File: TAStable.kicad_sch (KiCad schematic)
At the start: 12 parts, among them J1 Conn_01x06_Pin, U1 74HCT1G04, U2 CS2300-CP, U3 74LVC1G14

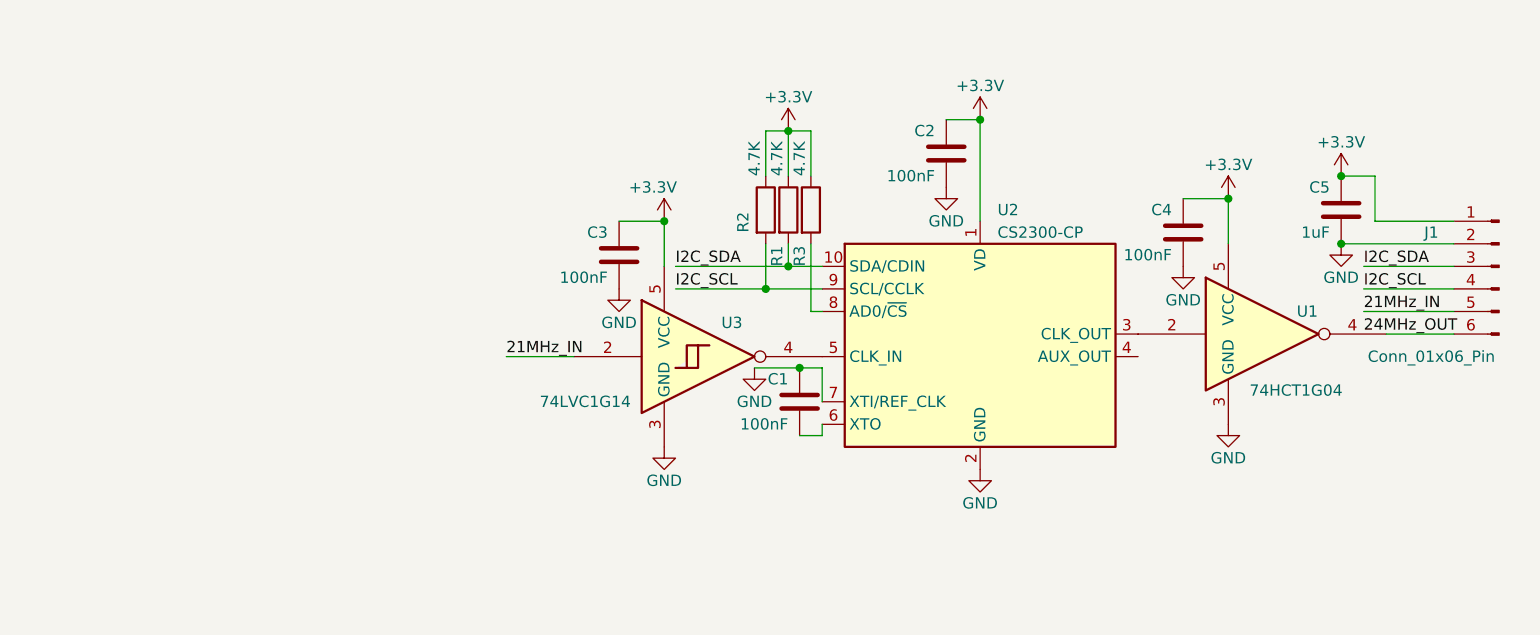
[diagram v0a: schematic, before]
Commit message: code!
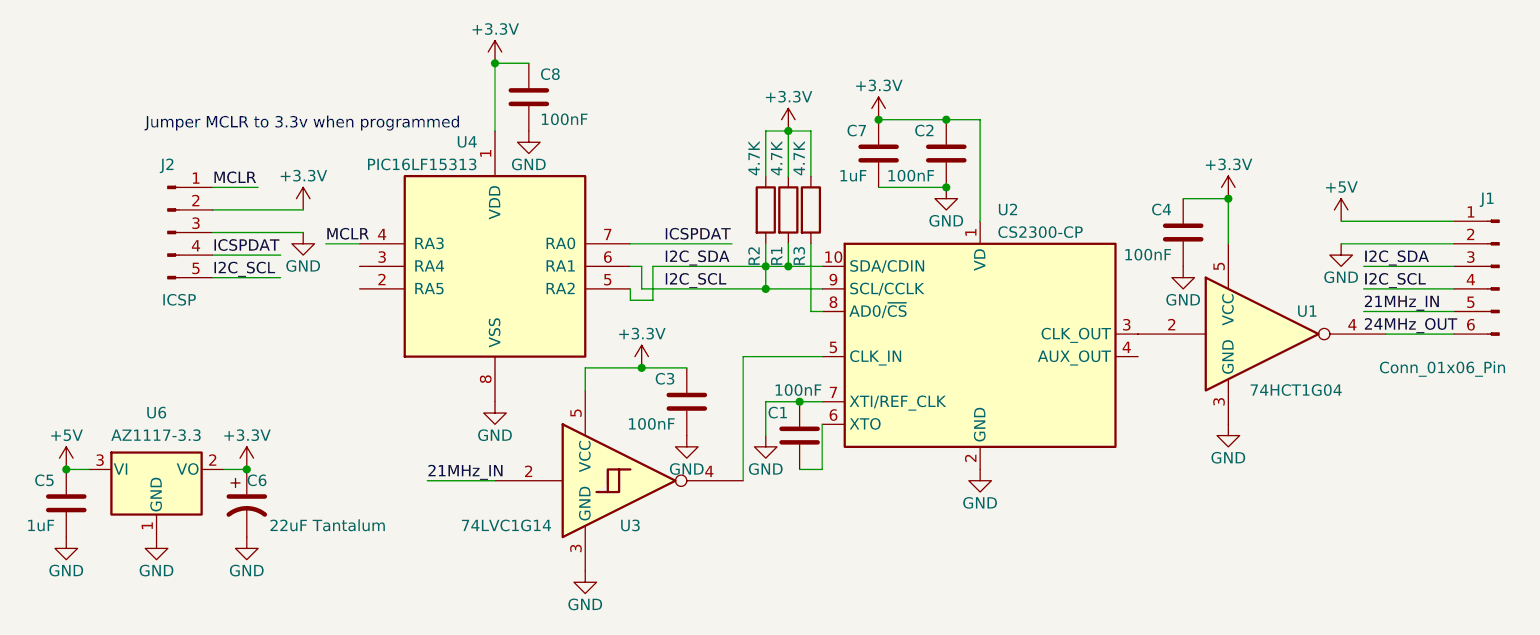
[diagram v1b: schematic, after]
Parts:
- added C6: 22uF Tantalum, Capacitor_SMD:C_1206_3216Metric, symbol Device:C_Polarized_US
- added C7: 1uF, Capacitor_SMD:C_0603_1608Metric, symbol Device:C
- added C8: 100nF, Capacitor_SMD:C_0603_1608Metric, symbol Device:C
- added J2: ICSP, Connector_PinSocket_2.54mm:PinSocket_1x05_P2.54mm_Vertical, symbol Connector:Conn_01x05_Pin
- added U4: PIC16LF15313, Package_SO:SOIC-8_3.9x4.9mm_P1.27mm, symbol MCU_Microchip_PIC12:PIC12F1501-IMS
- added U6: AZ1117-3.3, Package_TO_SOT_SMD:SOT-89-3, symbol Regulator_Linear:AZ1117-3.3
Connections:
- net I2C_SDA is gone; now on net I2C_SCL: J1.3 (Pin_3), R1.2, U2.10 (SDA/CDIN)
- net +3.3V: now also C6.1, C7.1, C8.1, J2.2 (Pin_2), U4.1 (VDD), U6.2 (VO); no longer C5.1, J1.1 (Pin_1)
- net GND: now also C6.2, C7.2, C8.2, J2.3 (Pin_3), U4.8 (VSS), U6.1 (GND)
- net I2C_SCL: now also J2.5 (Pin_5), U4.5 (RA2), U4.6 (RA1)
- new net +5V: C5.1, J1.1 (Pin_1), U6.3 (VI)
- new net ICSPDAT: J2.4 (Pin_4), U4.7 (RA0)
- new net MCLR: J2.1 (Pin_1), U4.4 (RA3)
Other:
- note added: "Jumper MCLR to 3.3v when programmed"
- moved on the sheet: C1, C3, U3
